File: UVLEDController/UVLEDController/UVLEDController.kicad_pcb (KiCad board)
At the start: 2 copper layers, 80 x 56 mm, 13 parts, among them J1-LED1 Screw_Terminal_01x02, J2-PWR1 Screw_Terminal_01x02, J3 Conn_01x04_Male, Q1 Q_NMOS_GDS

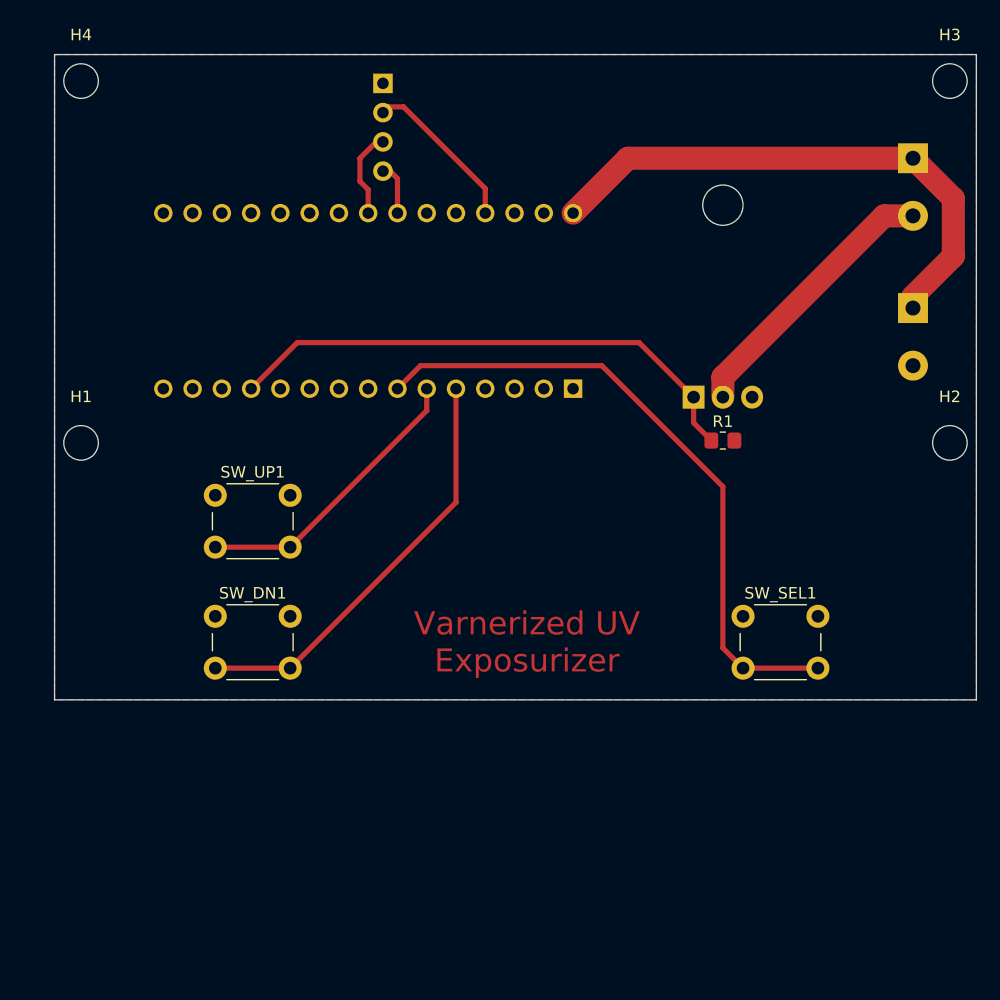
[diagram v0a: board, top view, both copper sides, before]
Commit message: Rotated.
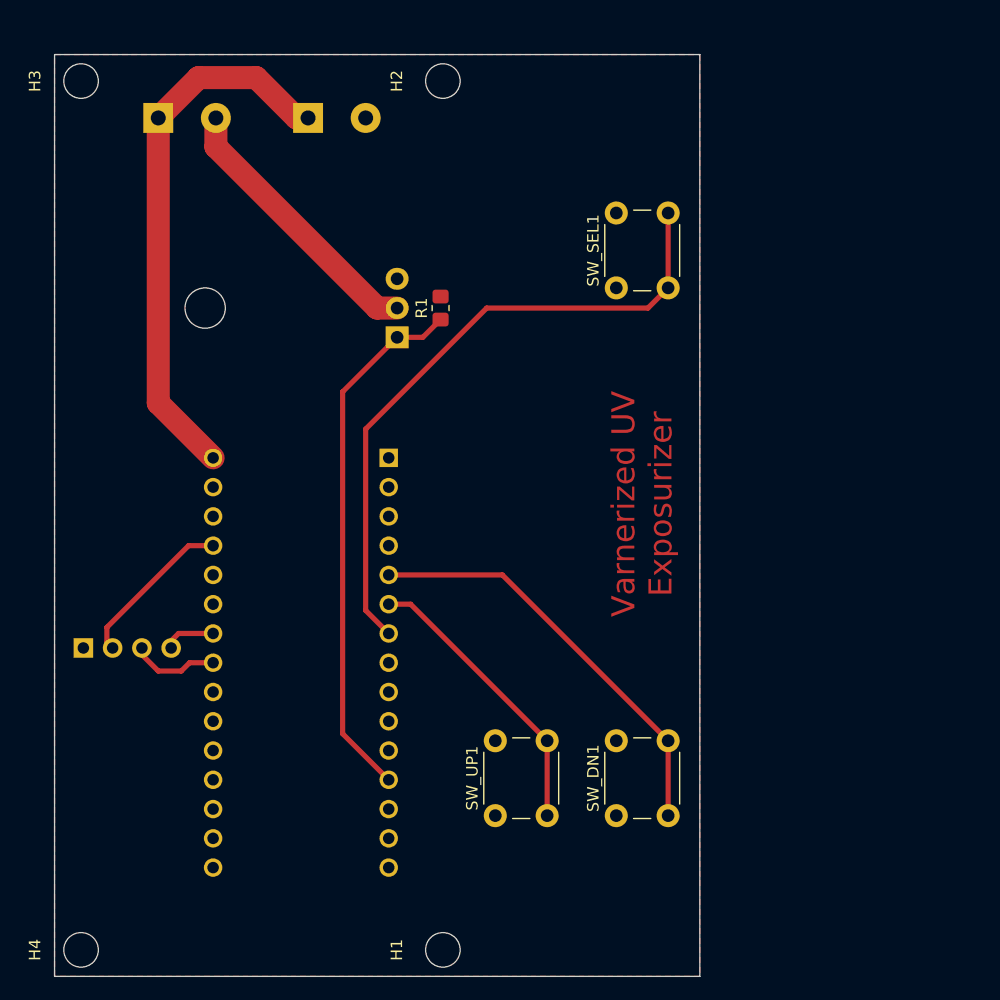
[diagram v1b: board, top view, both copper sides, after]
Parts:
- moved H4 75.4 mm to (122.3, 107.7), turned to 90 degrees
- moved H3 75.4 mm to (122.3, 32.3), turned to 90 degrees
- moved J1-LED1 65.6 mm to (129.0, 35.5), turned to 0 degrees
- moved J3 55.5 mm to (122.5, 81.5), turned to -90 degrees
- moved J2-PWR1 55.0 mm to (142.0, 35.5), turned to 0 degrees
- moved H1 54.1 mm to (153.7, 107.7), turned to 90 degrees
- moved H2 54.1 mm to (153.7, 32.3), turned to 90 degrees
- moved SW_DN1 38.9 mm to (168.8, 96.0), turned to 90 degrees
- moved SW_UP1 36.9 mm to (158.2, 96.0), turned to 90 degrees
- moved SW_SEL1 30.5 mm to (168.8, 50.2), turned to 90 degrees
- moved R1 27.1 mm to (153.5, 52.0), turned to 90 degrees
- moved Q1 26.2 mm to (149.7, 54.5), turned to 90 degrees
- moved A1 17.1 mm to (149.0, 65.0), turned to 180 degrees
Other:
- board size 80 x 56 mm -> 56 x 80 mm
